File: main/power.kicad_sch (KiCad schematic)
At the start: 7 parts, among them J3 USB_B_Micro, J4 Screw_Terminal_01x02

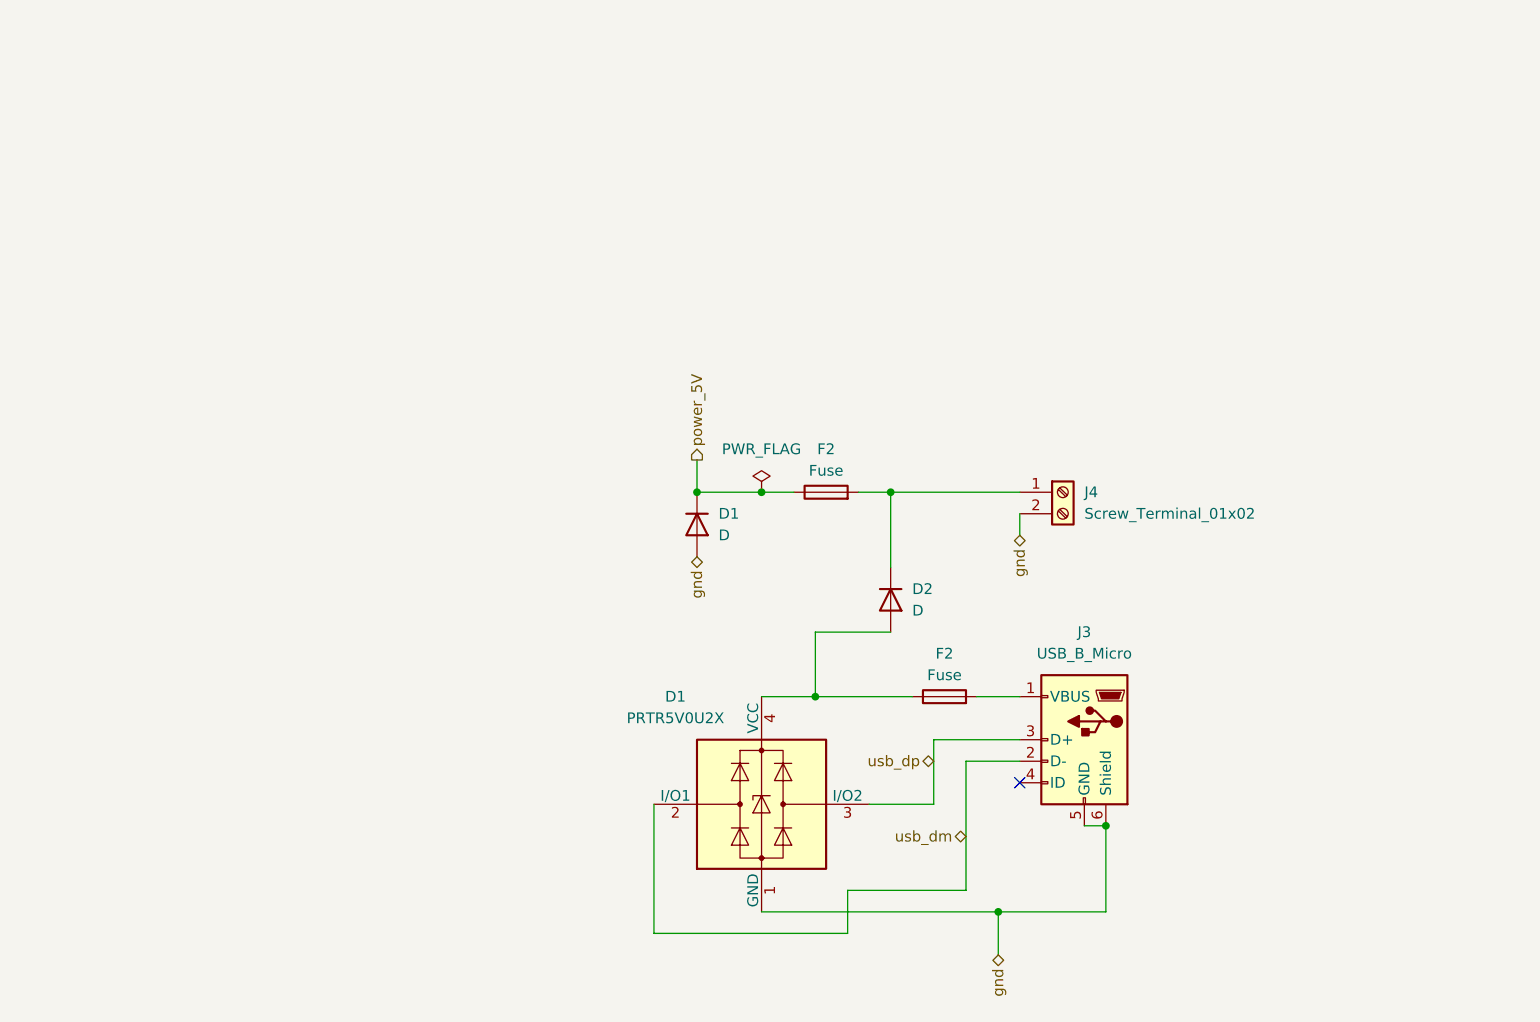
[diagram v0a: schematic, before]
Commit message: Power supply moved to battery
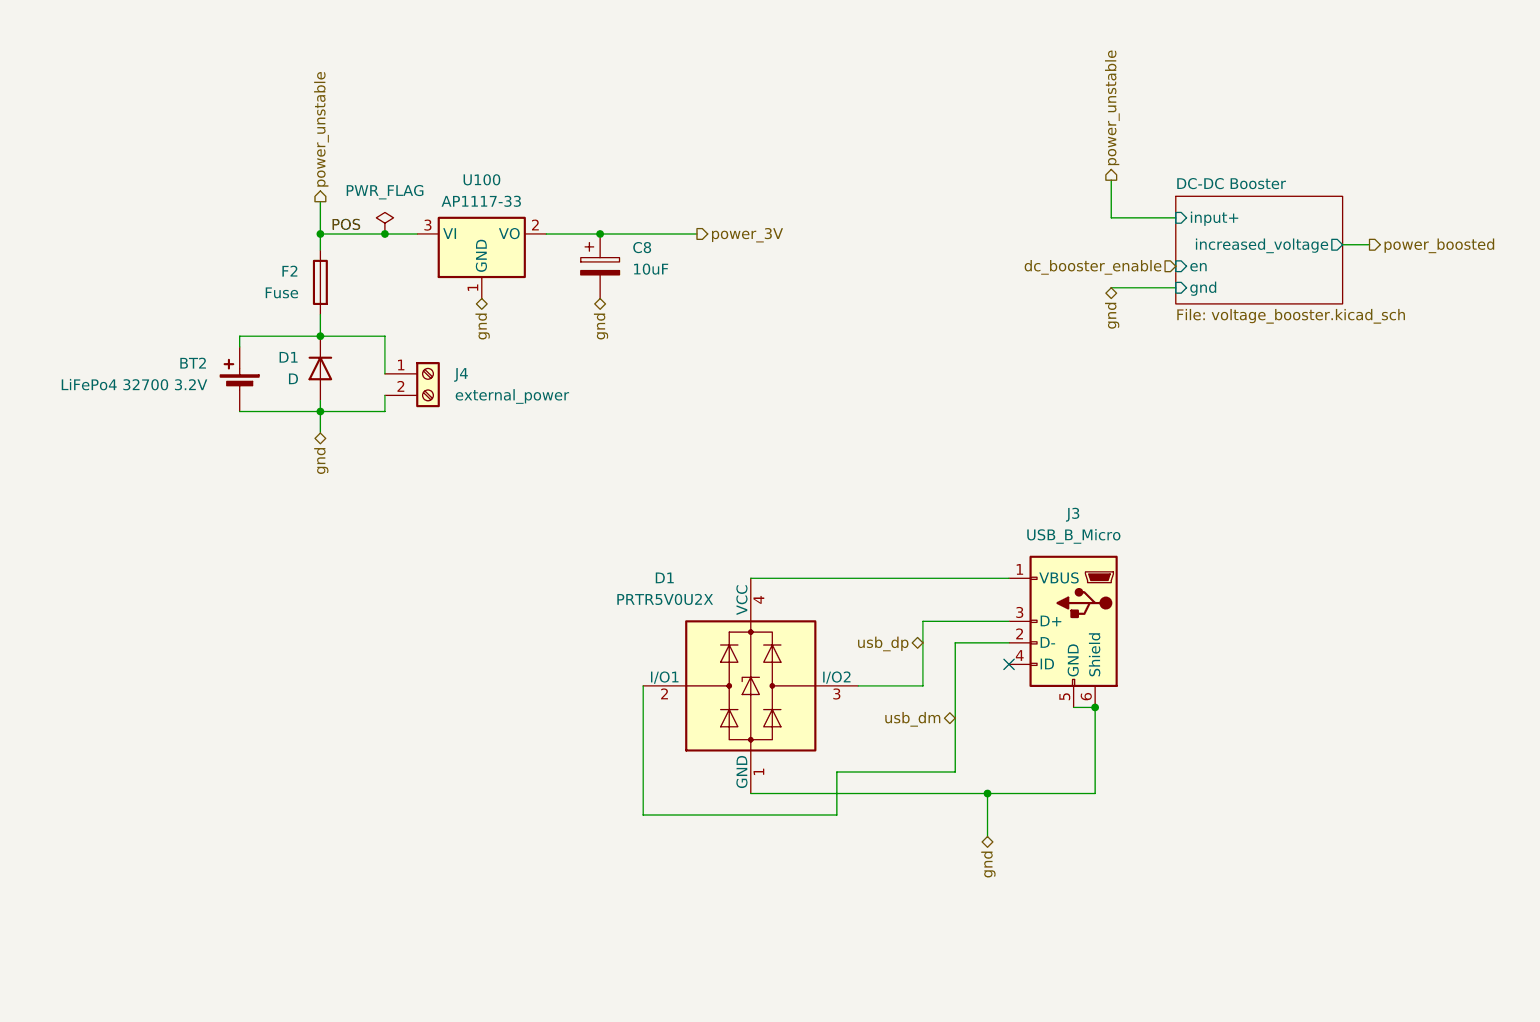
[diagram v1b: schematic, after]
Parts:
- removed D2: D, symbol Device:D
- removed F2: Fuse, symbol Device:Fuse
- added BT2: LiFePo4 32700 3.2V, symbol Device:Battery_Cell
- added C8: 10uF, symbol Device:C_Polarized
- added U100: AP1117-33, Package_TO_SOT_SMD:SOT-223-3_TabPin2, symbol Regulator_Linear:AP1117-33
- J4: value Screw_Terminal_01x02 -> external_power
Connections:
- net gnd: now also BT2.2 (-), C8.2, U100.1 (GND)
- net at F2.2, J4.1 (Pin_1): now also D1.1 (K), BT2.1 (+)
- net at D1.4 (VCC): now also J3.1 (VBUS)
- net power_5V renamed power_unstable
- net power_unstable: now also U100.3 (VI); no longer D1.1 (K)
- new net power_3V: C8.1, U100.2 (VO)
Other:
- added sheet DC-DC Booster (voltage_booster.kicad_sch)
- moved on the sheet: D1, F2, J3, J4
